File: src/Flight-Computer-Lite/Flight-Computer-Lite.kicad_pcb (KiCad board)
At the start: 4 copper layers, 88.4 x 33.9 mm, 75 parts, among them J1 Jumper_NO, J2 Jumper_NO, P1 1546551-2, P2 3220-20-0200-00, P3 USB, P4 1984659, Q1 QS5U17TR, Q2 QS5U17TR, U1 STM32H750VBTx, U2 LMS8117AMP-3.3_NOPB, U3 SST25VF040B-50-4I-S2AE-T, U4 CP2102-GMR(QFN28), U5 TS391IYLT, U6 BMP390, U7 TS391IYLT, U8 TS391IYLT, Y1 ECS-240-18-33-JGN-TR

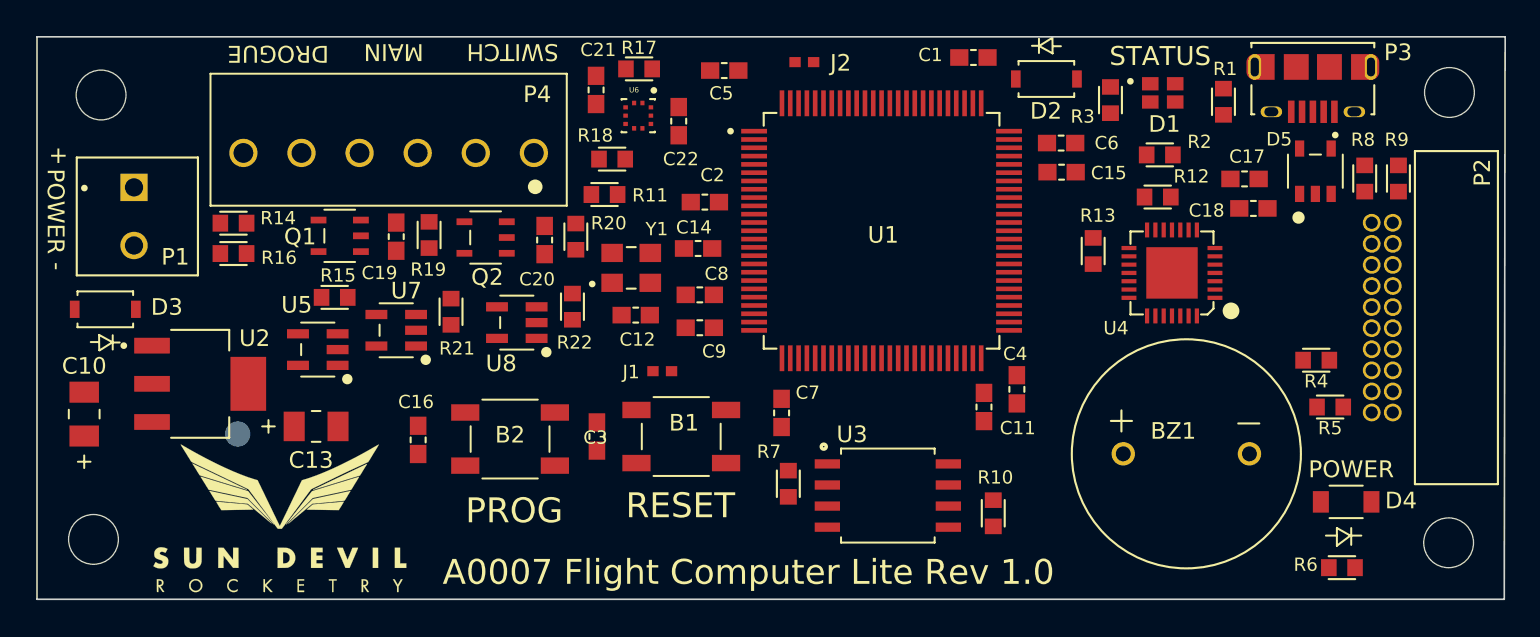
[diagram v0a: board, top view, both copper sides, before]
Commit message: finalized rev1 routing
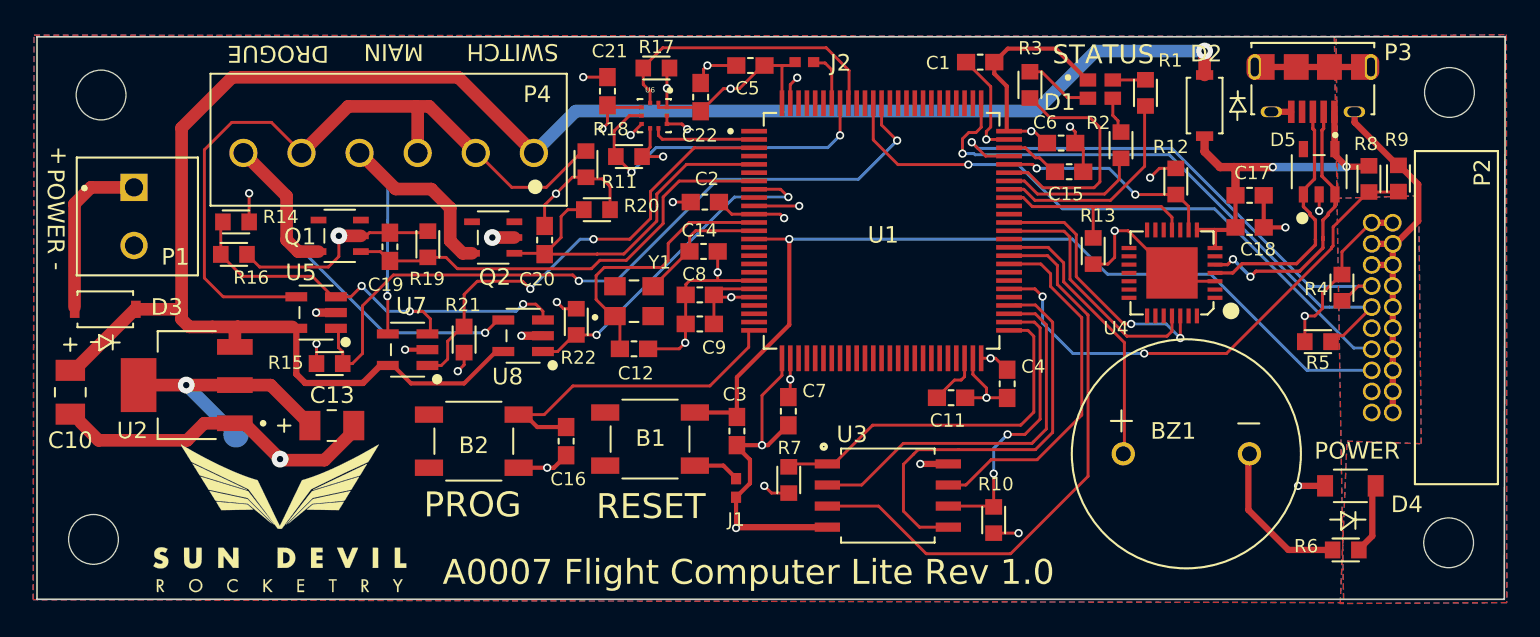
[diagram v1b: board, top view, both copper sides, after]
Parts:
- moved D2 9.67 mm to (221.2, 80.6), turned to -90 degrees
- moved C16 8.92 mm to (182.7, 100.9), turned to -90 degrees
- moved C3 8.44 mm to (193.0, 100.3), turned to -90 degrees
- moved J1 8.32 mm to (192.9, 103.7), turned to 90 degrees
- moved R3 4.94 mm to (210.6, 79.4)
- moved R1 4.73 mm to (217.6, 79.9)
- moved R4 4.64 mm to (229.4, 91.6), turned to 90 degrees
- moved R5 4.01 mm to (228.0, 94.9)
- moved R15 4.00 mm to (168.5, 96.2)
- moved D1 3.77 mm to (214.9, 79.7)
- moved R2 2.41 mm to (216.1, 83.0), turned to 90 degrees
- moved U5 2.23 mm to (167.6, 93.1)
- moved B2 2.19 mm to (177.1, 100.9), turned to 180 degrees
- moved R11 2.14 mm to (183.9, 84.2), turned to 90 degrees
- moved R20 2.06 mm to (184.6, 86.9), turned to 180 degrees
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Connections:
- U1 pad 25: unconnected-(U1-Pad25) -> PROG
- U1 pad 45: PROG -> unconnected-(U1-Pad45)
- U1 pad 5: unconnected-(U1-Pad5) -> MAIN
- U1 pad 59: ~{FLASH_WP} -> ~{FLASH_HOLD}
- U1 pad 60: ~{FLASH_HOLD} -> ~{FLASH_WP}
- U1 pad 87: MAIN -> unconnected-(U1-Pad87)
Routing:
- net Earth: track 0.00 -> 161.8 mm, vias 0 -> 26
- net VIN: track 0.00 -> 112.8 mm, vias 0 -> 1
- net 3.3V: track 0.00 -> 81.9 mm, vias 0 -> 19
- net NRST: track 0.00 -> 55.1 mm, vias 0 -> 1
- net ~{SWITCH}: track 0.00 -> 45.9 mm, vias 0 -> 2
- net VIN_SW: track 0.00 -> 44.5 mm
- net SWO: track 0.00 -> 37.2 mm, vias 0 -> 1
- net ~{FLASH_WP}: track 0.00 -> 35.5 mm
- net SWCLK: track 0.00 -> 34.9 mm, vias 0 -> 1
- net SWDIO: track 0.00 -> 32.2 mm, vias 0 -> 1
- net USB_DETECT: track 0.00 -> 30.7 mm, vias 0 -> 2
- net Net-(P4-Pad6): track 0.00 -> 30.2 mm, vias 0 -> 1
- net ~{MAIN_CONT}: track 0.00 -> 27.8 mm, vias 0 -> 2
- net DROGUE: track 0.00 -> 26.7 mm
- net VCOMP: track 0.00 -> 26.0 mm, vias 0 -> 3
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- added copper zone on In2.Cu, net 3.3V
- added copper zone on B.Cu, net Earth
- added copper zone on F.Cu, net Earth
- added copper zone on In1.Cu, net Earth
